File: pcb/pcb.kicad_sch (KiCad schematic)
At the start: 38 parts, among them J1 Conn_01x04, SW1 SW_Push, SW10 SW_Push, SW11 SW_Push, SW12 SW_Push, SW2 SW_Push, SW3 SW_Push, SW4 SW_Push, SW5 SW_Push, SW6 SW_Push, SW7 SW_Push, SW8 SW_Push, SW9 SW_Push, U1 XIAO-RP2040-DIP

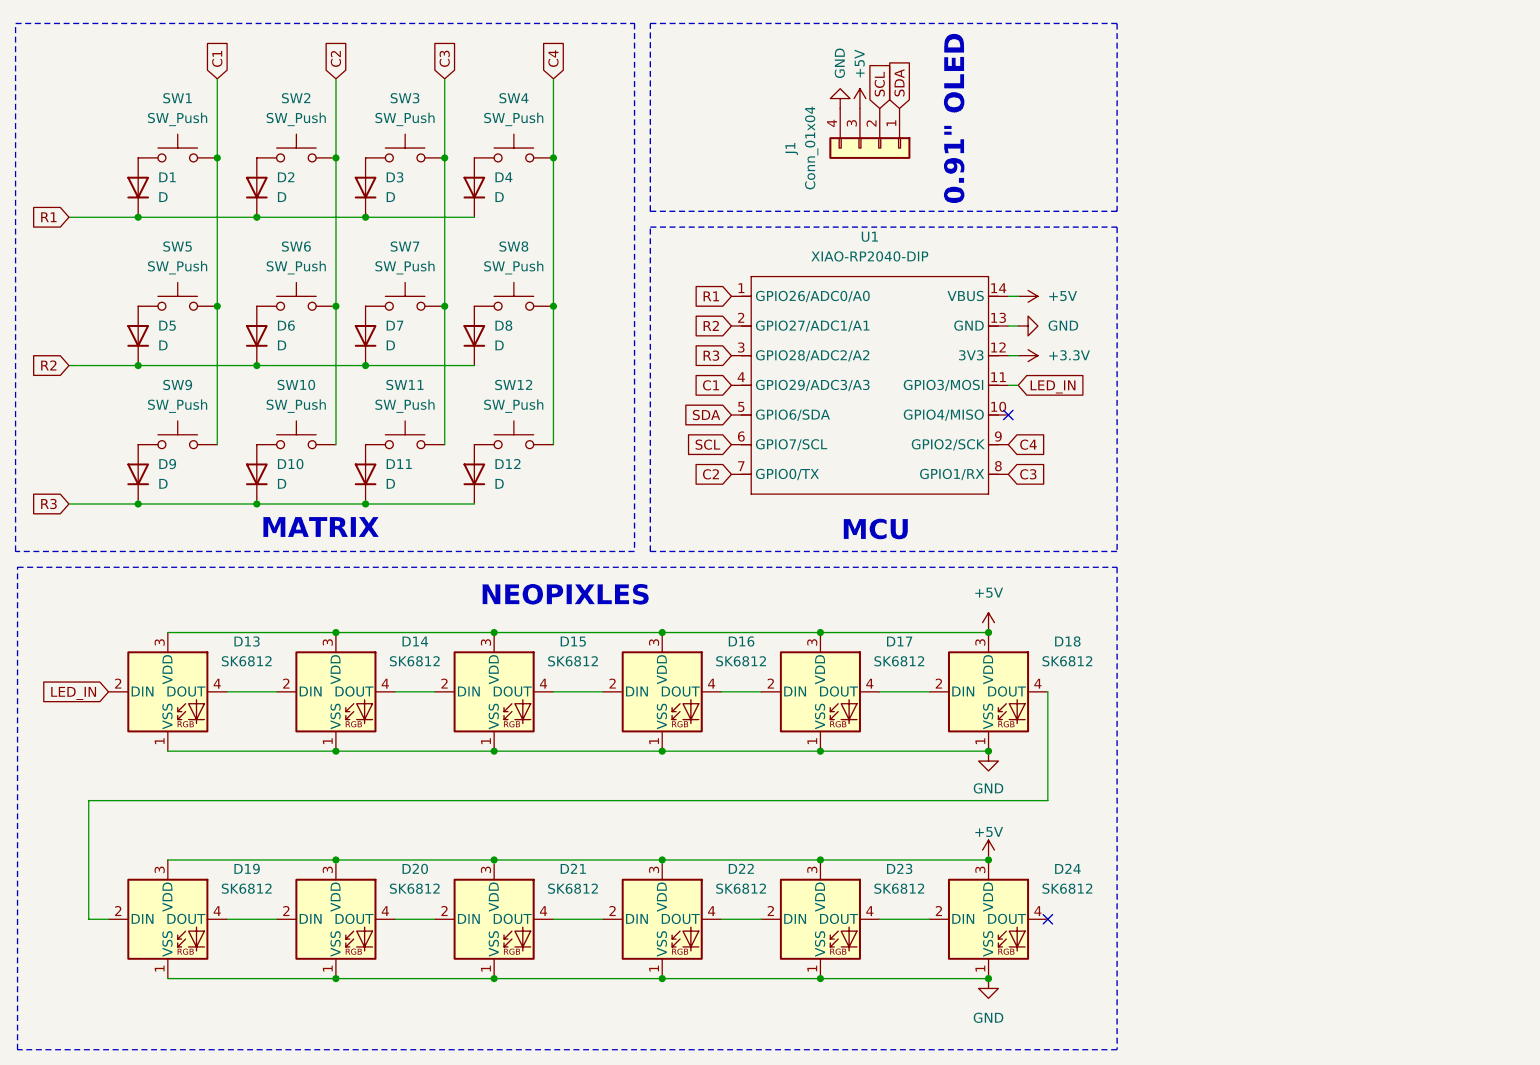
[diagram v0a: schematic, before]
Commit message: Updated the PCB files
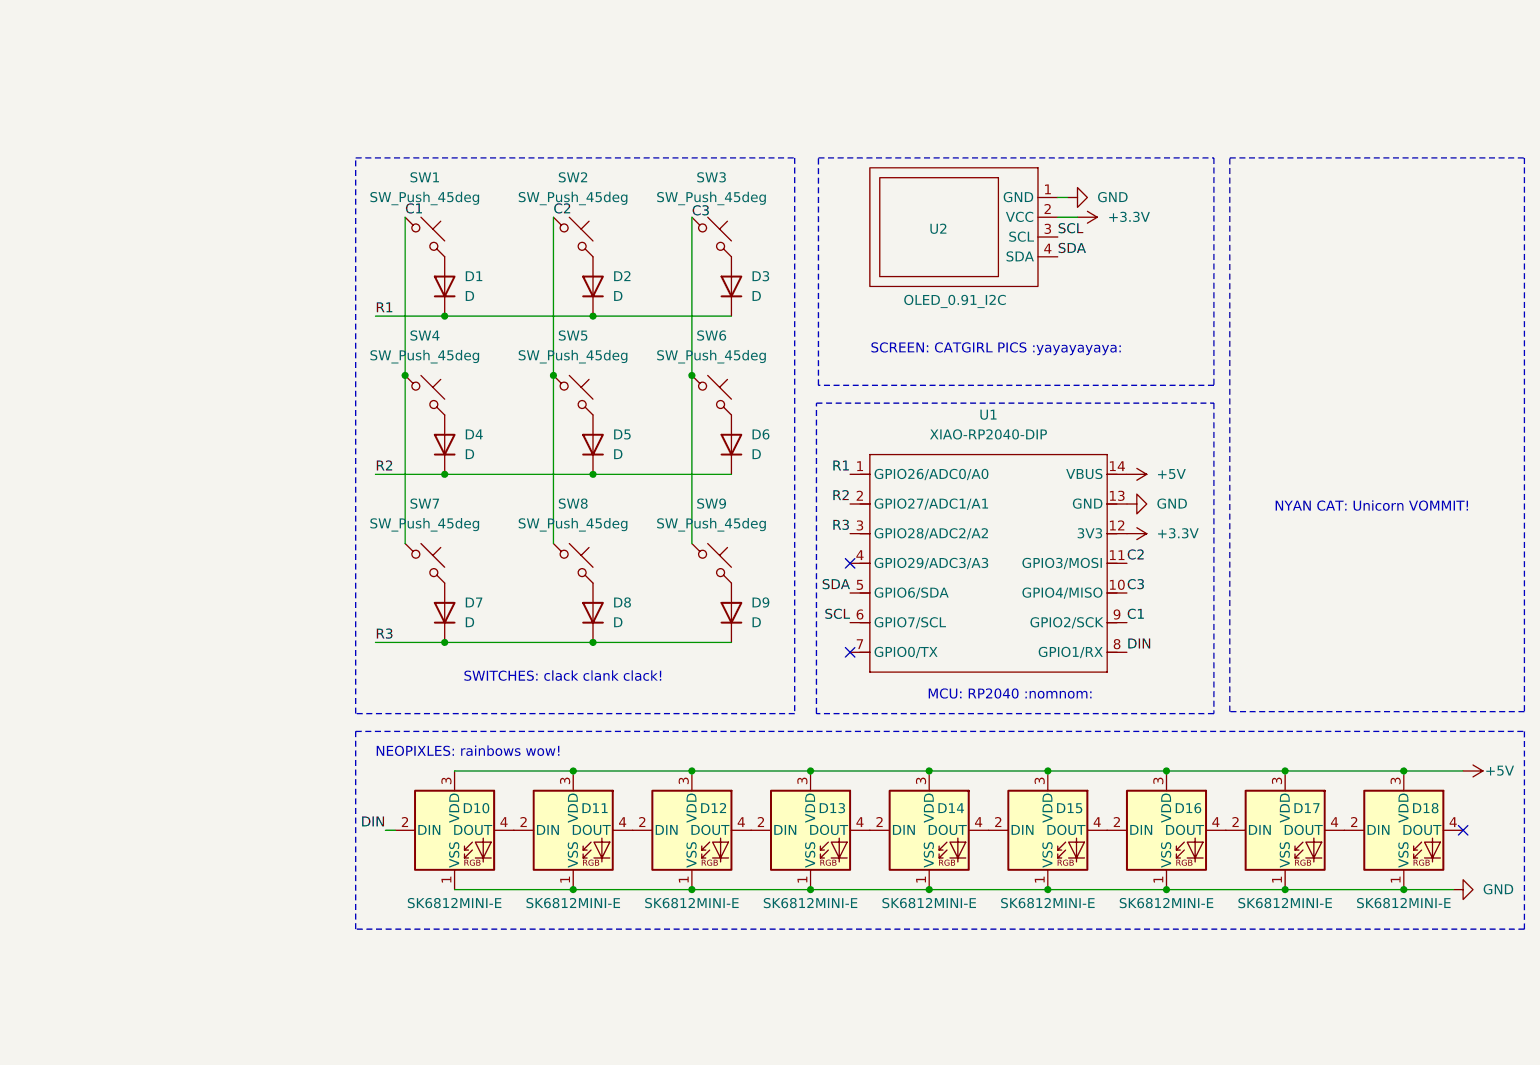
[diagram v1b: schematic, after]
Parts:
- removed D10, D11, D12: D, Diode_THT:D_DO-35_SOD27_P7.62mm_Horizontal, symbol Device:D
- removed D13, D14, D15, D16, D17, D18, D19, D20, D21, D22, D23, D24: SK6812, KEYS:MX_SK6812MINI-E, symbol LED:SK6812
- removed J1: Conn_01x04, Connector_PinHeader_2.54mm:PinHeader_1x04_P2.54mm_Vertical, symbol Connector_Generic:Conn_01x04
- removed SW1, SW10, SW11, SW12, SW2, SW3, SW4, SW5, SW6, SW7, SW8, SW9: SW_Push, Button_Switch_Keyboard:SW_Cherry_MX_1.00u_PCB, symbol Switch:SW_Push
- added D10, D11, D12, D13, D14, D15, D16, D17, D18: SK6812MINI-E, SK6812 MINI-E:MX_SK6812MINI-E, symbol LED:SK6812MINI-E
- added SW1, SW2, SW3, SW4, SW5, SW6, SW7, SW8, SW9: SW_Push_45deg, KEYS:SW_Cherry_MX_PCB, symbol Switch:SW_Push_45deg
- added U2: OLED_0.91_I2C, Connector_PinSocket_2.54mm:PinSocket_1x04_P2.54mm_Vertical, symbol New_Library:0.91{dblquote}_I2C
- D1, D2, D3, D4, D5, D6, D7, D8, D9: footprint Diode_THT:D_DO-35_SOD27_P7.62mm_Horizontal -> Diode_SMD:D_SOD-123
- U1: footprint XIAO:XIAO-RP2040-DIP -> XIAO:XIAO-RP2040-SMD
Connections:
- net C4 is gone; now on net C1: U1.9 (GPIO2/SCK)
- net LED_IN is gone; now on net C2: U1.11 (GPIO3/MOSI)
- net +3.3V: now also U2.2 (VCC)
- net +5V: now also D10.3 (VDD), D11.3 (VDD), D12.3 (VDD), D13.3 (VDD), D14.3 (VDD), D15.3 (VDD), D16.3 (VDD), D17.3 (VDD), D18.3 (VDD)
- net C1: now also SW1.1, SW4.1, SW7.1; no longer U1.4 (GPIO29/ADC3/A3)
- net C2: now also SW2.1, SW5.1, SW8.1; no longer U1.7 (GPIO0/TX)
- net C3: now also U1.10 (GPIO4/MISO), SW3.1, SW6.1, SW9.1; no longer U1.8 (GPIO1/RX)
- net GND: now also D10.1 (VSS), D11.1 (VSS), D12.1 (VSS), D13.1 (VSS), D14.1 (VSS), D15.1 (VSS), D16.1 (VSS), D17.1 (VSS), D18.1 (VSS), U2.1 (GND)
- net R1: no longer D4.1 (K)
- net R2: now also D4.1 (K); no longer D7.1 (K), D8.1 (K)
- net R3: now also D7.1 (K), D8.1 (K)
- net SCL: now also U2.3 (SCL)
- net SDA: now also U2.4 (SDA)
- net at D4.2 (A): now also SW4.2
- net at D1.2 (A): now also SW1.2
- net at D2.2 (A): now also SW2.2
- net at D3.2 (A): now also SW3.2
- net at D5.2 (A): now also SW5.2
- net at D7.2 (A): now also SW7.2
- net at D8.2 (A): now also SW8.2
- net at D9.2 (A): now also SW9.2
- net at D6.2 (A): now also SW6.2
- new net: D15.4 (DOUT), D16.2 (DIN)
- new net: D16.4 (DOUT), D17.2 (DIN)
- new net: D10.4 (DOUT), D11.2 (DIN)
- new net: D11.4 (DOUT), D12.2 (DIN)
- new net: D14.4 (DOUT), D15.2 (DIN)
- new net: D12.4 (DOUT), D13.2 (DIN)
- new net: D13.4 (DOUT), D14.2 (DIN)
- new net: D17.4 (DOUT), D18.2 (DIN)
- new net DIN: D10.2 (DIN), U1.8 (GPIO1/RX)
- no-connect marks 2 -> 3
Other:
- note added: "MCU: RP2040 :nomnom:"
- note added: "NEOPIXLES: rainbows wow!"
- note added: "NYAN CAT: Unicorn VOMMIT!"
- note added: "SCREEN: CATGIRL PICS :yayayayaya:"
- note added: "SWITCHES: clack clank clack!"
- note removed: "0.91" OLED"
- note removed: "MATRIX"
- note removed: "MCU"
- note removed: "NEOPIXLES"
